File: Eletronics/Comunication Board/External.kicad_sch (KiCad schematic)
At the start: 5 parts, among them J2 Conn_01x14_Socket

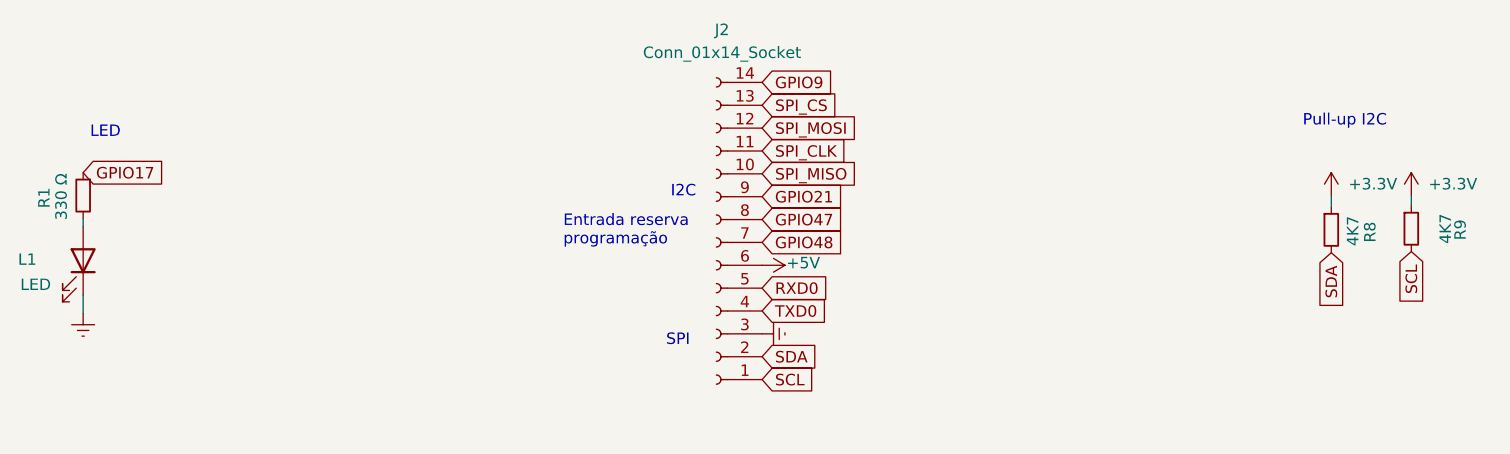
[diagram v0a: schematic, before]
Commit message: Communication Board edit
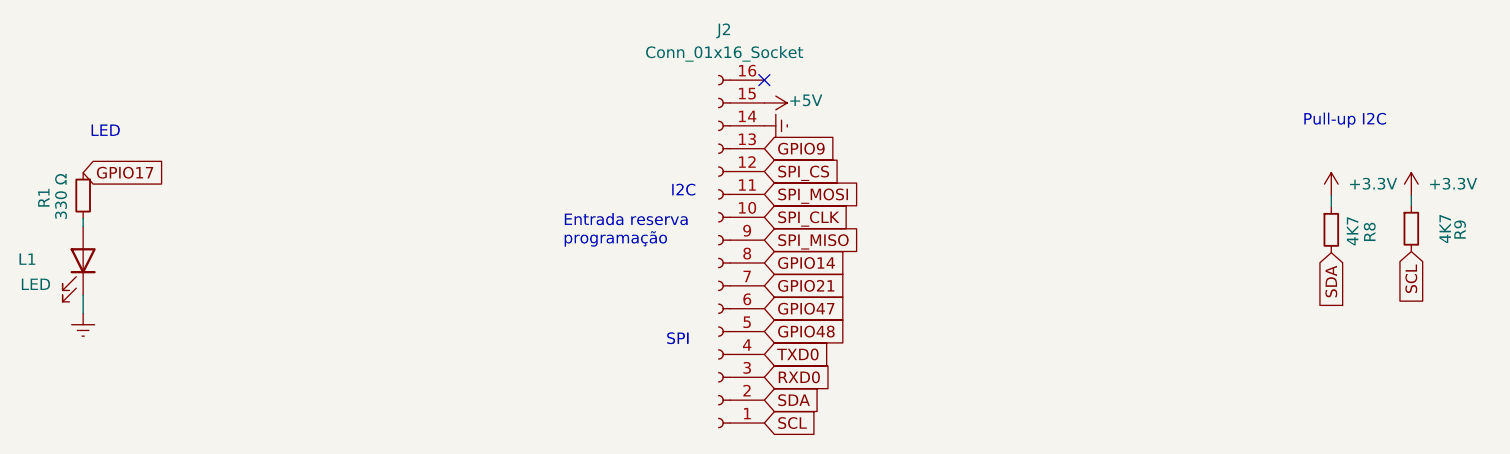
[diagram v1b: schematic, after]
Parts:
- removed J2: Conn_01x14_Socket, Connector_IDC:IDC-Header_2x07_P2.54mm_Vertical, symbol Connector:Conn_01x14_Socket
- added J2: Conn_01x16_Socket, Connector_IDC:IDC-Header_2x08_P2.54mm_Vertical, symbol Connector:Conn_01x16_Socket
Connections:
- net +5V: now also J2.15 (Pin_15)
- net GNDREF: now also J2.14 (Pin_14)
- net GPIO21: now also J2.7 (Pin_7)
- net GPIO47: now also J2.6 (Pin_6)
- net GPIO48: now also J2.5 (Pin_5)
- net GPIO9: now also J2.13 (Pin_13)
- net RXD0: now also J2.3 (Pin_3)
- net SCL: now also J2.1 (Pin_1)
- net SDA: now also J2.2 (Pin_2)
- net SPI_CLK: now also J2.10 (Pin_10)
- net SPI_CS: now also J2.12 (Pin_12)
- net SPI_MISO: now also J2.9 (Pin_9)
- net SPI_MOSI: now also J2.11 (Pin_11)
- net TXD0: now also J2.4 (Pin_4)
- new net GPIO14: J2.8 (Pin_8)
- no-connect marks 0 -> 1
